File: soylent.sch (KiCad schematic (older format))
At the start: 24 parts, among them J1 DB9_Female, J2 Conn_01x04, J3 Conn_01x04, J4 Conn_02x03_Counter_Clockwise, Q1 BC847BPN, Q2 BC847BPN, U1 ATtiny202-SS, U2 MIC5504-3.3YM5

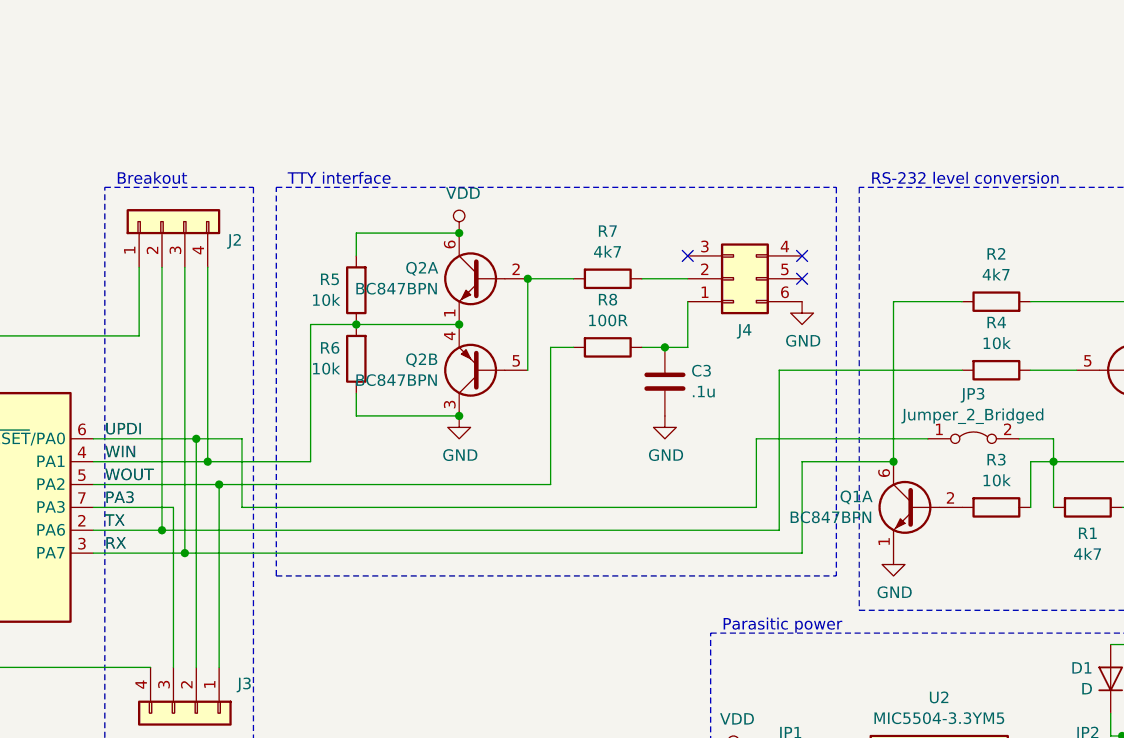
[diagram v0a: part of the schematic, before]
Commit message: Making more room on the schematic
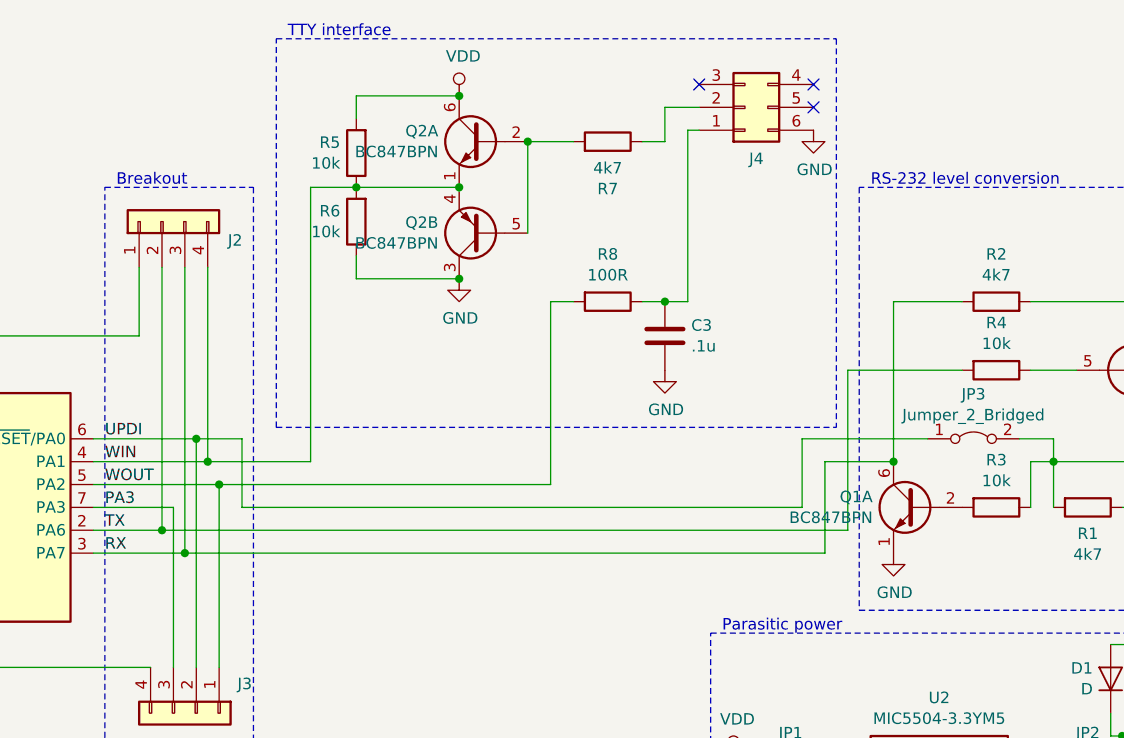
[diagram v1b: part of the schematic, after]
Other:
- moved on the sheet: C3, J4, Q2A, Q2B, R5, R6, R7, R8
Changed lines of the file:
@@
 Connection ~ 3750 3900
 Wire Wire Line
-	6550 4000 6550 3600
-Wire Wire Line
-	6550 3600 6950 3600
+	6650 4000 6650 3600
+Wire Wire Line
+	6650 3600 6950 3600
 Connection ~ 3850 4000
 Wire Wire Line
@@
 Parasitic power
 Wire Notes Line
-	6700 2400 6700 4100
-Wire Notes Line
-	4250 4100 4250 2400
-Wire Wire Line
-	6450 3900 6450 3200
-Wire Wire Line
-	6450 3200 7250 3200
+	6700 1750 6700 3450
+Wire Notes Line
+	4250 3450 4250 1750
+Wire Wire Line
+	6750 3900 6750 3200
+Wire Wire Line
+	6750 3200 7250 3200
 Wire Wire Line
 	7550 3200 7750 3200
-Text Notes 4300 2400 0    50   ~ 0
+Text Notes 4300 1750 0    50   ~ 0
 TTY interface
 $Comp
 L power:GND #PWR0108
 U 1 1 5DEFD9EC
-P 6550 2900
-F 0 "#PWR0108" H 6550 2650 50  0001 C CNN
-F 1 "GND" H 6555 2727 50  0000 C CNN
-F 2 "" H 6550 2900 50  0001 C CNN
-F 3 "" H 6550 2900 50  0001 C CNN
-	1    6550 2900
+P 6600 2150
+F 0 "#PWR0108" H 6600 1900 50  0001 C CNN
+F 1 "GND" H 6605 1977 50  0000 C CNN
+F 2 "" H 6600 2150 50  0001 C CNN
+F 3 "" H 6600 2150 50  0001 C CNN
+	1    6600 2150
 	1    0    0    -1
 $EndComp
@@
 L Device:R R7
 U 1 1 5DEFDFE7
-P 5700 2800
-F 0 "R7" V 5493 2800 50  0000 C CNN
-F 1 "4k7" V 5584 2800 50  0000 C CNN
-F 2 "Resistors_SMD:R_0603_HandSoldering" V 5630 2800 50  0001 C CNN
-F 3 "~" H 5700 2800 50  0001 C CNN
-	1    5700 2800
-	0    1    1    0
+P 5700 2200
+F 0 "R7" V 5493 2200 50  0000 C CNN
+F 1 "4k7" V 5584 2200 50  0000 C CNN
+F 2 "Resistors_SMD:R_0603_HandSoldering" V 5630 2200 50  0001 C CNN
+F 3 "~" H 5700 2200 50  0001 C CNN
+	1    5700 2200
+	0    1    -1   0
 $EndComp
 $Comp
 L Transistor_BJT:BC847BPN Q2
 U 2 1 5DF05573
-P 5150 3200
-F 0 "Q2" H 5341 3154 50  0000 L CNN
-F 1 "BC847BPN" H 5341 3245 50  0000 L CNN
-F 2 "TO_SOT_Packages_SMD:SOT-363_SC-70-6_Handsoldering" H 5350 3300 50  0001 C CNN
-F 3 "https://assets.nexperia.com/documents/data-sheet/BC847BPN.pdf" H 5150 3200 50  0001 C CNN
-	2    5150 3200
+P 5150 2600
+F 0 "Q2" H 5341 2554 50  0000 L CNN
+F 1 "BC847BPN" H 5341 2645 50  0000 L CNN
+F 2 "TO_SOT_Packages_SMD:SOT-363_SC-70-6_Handsoldering" H 5350 2700 50  0001 C CNN
+F 3 "https://assets.nexperia.com/documents/data-sheet/BC847BPN.pdf" H 5150 2600 50  0001 C CNN
+	2    5150 2600
 	-1   0    0    1
 $EndComp
@@
 L Transistor_BJT:BC847BPN Q2
 U 1 1 5DF18897
-P 5150 2800
-F 0 "Q2" H 5341 2846 50  0000 L CNN
-F 1 "BC847BPN" H 5341 2755 50  0000 L CNN
-F 2 "TO_SOT_Packages_SMD:SOT-363_SC-70-6_Handsoldering" H 5350 2900 50  0001 C CNN
-F 3 "https://assets.nexperia.com/documents/data-sheet/BC847BPN.pdf" H 5150 2800 50  0001 C CNN
-	1    5150 2800
+P 5150 2200
+F 0 "Q2" H 5341 2246 50  0000 L CNN
+F 1 "BC847BPN" H 5341 2155 50  0000 L CNN
+F 2 "TO_SOT_Packages_SMD:SOT-363_SC-70-6_Handsoldering" H 5350 2300 50  0001 C CNN
+F 3 "https://assets.nexperia.com/documents/data-sheet/BC847BPN.pdf" H 5150 2200 50  0001 C CNN
+	1    5150 2200
 	-1   0    0    -1
 $EndComp
 Wire Wire Line
-	3750 3900 6450 3900
-Wire Wire Line
-	3850 4000 6550 4000
-Wire Notes Line
-	4250 2400 6700 2400
-Wire Notes Line
-	4250 4100 6700 4100
+	3750 3900 6750 3900
+Wire Wire Line
+	3850 4000 6650 4000
+Wire Notes Line
+	4250 1750 6700 1750
+Wire Notes Line
+	4250 3450 6700 3450
 Wire Wire Line
 	3900 3500 4100 3500
@@
 	4100 3500 4100 3800
 Wire Wire Line
-	4100 3800 6350 3800
-Wire Wire Line
-	6350 3800 6350 3500
-Wire Wire Line
-	6350 3500 7100 3500
+	4100 3800 6550 3800
+Wire Wire Line
+	6550 3800 6550 3500
+Wire Wire Line
+	6550 3500 7100 3500
 Connection ~ 3900 3500
 $Comp
 L power:VDD #PWR0109
 U 1 1 5DF48DE3
-P 5050 2600
-F 0 "#PWR0109" H 5050 2450 50  0001 C CNN
-F 1 "VDD" H 5068 2773 50  0000 C CNN
-F 2 "" H 5050 2600 50  0001 C CNN
-F 3 "" H 5050 2600 50  0001 C CNN
-	1    5050 2600
-	1    0    0    -1
-$EndComp
-$Comp
-L power:GND #PWR0110
-U 1 1 5DF492BB
-P 5050 3400
-F 0 "#PWR0110" H 5050 3150 50  0001 C CNN
-F 1 "GND" H 5055 3227 50  0000 C CNN
-F 2 "" H 5050 3400 50  0001 C CNN
-F 3 "" H 5050 3400 50  0001 C CNN
-	1    5050 3400
-	1    0    0    -1
-$EndComp
-Wire Wire Line
-	5050 3000 4600 3000
-Connection ~ 5050 3000
-Wire Wire Line
-	5350 3200 5350 2800
-Wire Wire Line
-	5350 2800 5550 2800
-Connection ~ 5350 2800
-Wire Wire Line
-	5850 2800 6050 2800
+P 5050 2000
+F 0 "#PWR0109" H 5050 1850 50  0001 C CNN
+F 1 "VDD" H 5068 2173 50  0000 C CNN
+F 2 "" H 5050 2000 50  0001 C CNN
+F 3 "" H 5050 2000 50  0001 C CNN
+	1    5050 2000
+	1    0    0    -1
+$EndComp
+Wire Wire Line
+	5050 2400 4600 2400
+Connection ~ 5050 2400
+Wire Wire Line
+	5350 2600 5350 2200
+Wire Wire Line
+	5350 2200 5550 2200
+Connection ~ 5350 2200
 $Comp
 L Device:R R5
 U 1 1 5DF5183F
-P 4600 2850
-F 0 "R5" H 4670 2804 50  0000 L CNN
-F 1 "10k" H 4670 2895 50  0000 L CNN
-F 2 "Resistors_SMD:R_0603_HandSoldering" V 4530 2850 50  0001 C CNN
-F 3 "~" H 4600 2850 50  0001 C CNN
-	1    4600 2850
+P 4600 2250
+F 0 "R5" H 4670 2204 50  0000 L CNN
+F 1 "10k" H 4670 2295 50  0000 L CNN
+F 2 "Resistors_SMD:R_0603_HandSoldering" V 4530 2250 50  0001 C CNN
+F 3 "~" H 4600 2250 50  0001 C CNN
+	1    4600 2250
 	-1   0    0    1
 $EndComp
@@
 L Device:R R6
 U 1 1 5DF52A36
-P 4600 3150
-F 0 "R6" H 4670 3104 50  0000 L CNN
-F 1 "10k" H 4670 3195 50  0000 L CNN
-F 2 "Resistors_SMD:R_0603_HandSoldering" V 4530 3150 50  0001 C CNN
-F 3 "~" H 4600 3150 50  0001 C CNN
-	1    4600 3150
+P 4600 2550
+F 0 "R6" H 4670 2504 50  0000 L CNN
+F 1 "10k" H 4670 2595 50  0000 L CNN
+F 2 "Resistors_SMD:R_0603_HandSoldering" V 4530 2550 50  0001 C CNN
+F 3 "~" H 4600 2550 50  0001 C CNN
+	1    4600 2550
 	-1   0    0    1
 $EndComp
-Connection ~ 4600 3000
-Wire Wire Line
-	5050 2600 4600 2600
-Wire Wire Line
-	4600 2600 4600 2700
-Connection ~ 5050 2600
-Wire Wire Line
-	5050 3400 4600 3400
-Wire Wire Line
-	4600 3400 4600 3300
-Connection ~ 5050 3400
+Connection ~ 4600 2400
+Wire Wire Line
+	5050 2000 4600 2000
+Wire Wire Line
+	4600 2000 4600 2100
+Connection ~ 5050 2000
+Wire Wire Line
+	5050 2800 4600 2800
+Wire Wire Line
+	4600 2800 4600 2700
 Wire Wire Line
 	8350 3700 8350 4400
@@
 	8250 4250 8250 2400
 Wire Wire Line
-	4400 3000 4600 3000
-NoConn ~ 6050 2700
-NoConn ~ 6550 2700
-NoConn ~ 6550 2800
+	4400 2400 4600 2400
+NoConn ~ 6100 1950
+NoConn ~ 6600 1950
+NoConn ~ 6600 2050
 $Comp
 L Connector_Generic:Conn_02x03_Counter_Clockwise J4
 U 1 1 5DDE85A2
-P 6250 2800
-F 0 "J4" H 6300 3025 50  0000 C CNN
-F 1 "Conn_02x03_Counter_Clockwise" V 6345 2980 50  0001 L CNN
-F 2 "Pin_Headers:Pin_Header_Straight_2x03_Pitch2.54mm" H 6250 2800 50  0001 C CNN
-F 3 "~" H 6250 2800 50  0001 C CNN
-	1    6250 2800
+P 6300 2050
+F 0 "J4" H 6350 2275 50  0000 C CNN
+F 1 "Conn_02x03_Counter_Clockwise" V 6395 2230 50  0001 L CNN
+F 2 "Pin_Headers:Pin_Header_Straight_2x03_Pitch2.54mm" H 6300 2050 50  0001 C CNN
+F 3 "~" H 6300 2050 50  0001 C CNN
+	1    6300 2050
 	1    0    0    1
 $EndComp
@@
 	3950 3600 4400 3600
 Connection ~ 3950 3600
-Wire Wire Line
-	4400 3600 4400 3000
 Connection ~ 4000 3700
 $Comp
 L Device:R R8
 U 1 1 5DFD8224
-P 5700 3100
-F 0 "R8" V 5493 3100 50  0000 C CNN
-F 1 "100R" V 5584 3100 50  0000 C CNN
-F 2 "Resistors_SMD:R_0603_HandSoldering" V 5630 3100 50  0001 C CNN
-F 3 "~" H 5700 3100 50  0001 C CNN
-	1    5700 3100
+P 5700 2900
+F 0 "R8" V 5493 2900 50  0000 C CNN
+F 1 "100R" V 5584 2900 50  0000 C CNN
+F 2 "Resistors_SMD:R_0603_HandSoldering" V 5630 2900 50  0001 C CNN
+F 3 "~" H 5700 2900 50  0001 C CNN
+	1    5700 2900
 	0    1    1    0
 $EndComp
-Wire Wire Line
-	5450 3700 5450 3100
-Wire Wire Line
-	5450 3100 5550 3100
-Wire Wire Line
-	4000 3700 5450 3700
 $Comp
 L Device:C C3
 U 1 1 5DFEE336
-P 5950 3250
-F 0 "C3" H 6065 3296 50  0000 L CNN
-F 1 ".1u" H 6065 3205 50  0000 L CNN
-F 2 "Capacitor_SMD:C_0603_1608Metric_Pad1.05x0.95mm_HandSolder" H 5988 3100 50  0001 C CNN
-F 3 "~" H 5950 3250 50  0001 C CNN
-	1    5950 3250
+P 5950 3050
+F 0 "C3" H 6065 3096 50  0000 L CNN
+F 1 ".1u" H 6065 3005 50  0000 L CNN
+F 2 "Capacitor_SMD:C_0603_1608Metric_Pad1.05x0.95mm_HandSolder" H 5988 2900 50  0001 C CNN
+F 3 "~" H 5950 3050 50  0001 C CNN
+	1    5950 3050
 	1    0    0    -1
 $EndComp
@@
 L power:GND #PWR0111
 U 1 1 5DFEEE43
-P 5950 3400
-F 0 "#PWR0111" H 5950 3150 50  0001 C CNN
-F 1 "GND" H 5955 3227 50  0000 C CNN
-F 2 "" H 5950 3400 50  0001 C CNN
-F 3 "" H 5950 3400 50  0001 C CNN
-	1    5950 3400
-	1    0    0    -1
-$EndComp
-Wire Wire Line
-	5850 3100 5950 3100
-Wire Wire Line
-	5950 3100 6050 3100
-Wire Wire Line
-	6050 3100 6050 2900
-Connection ~ 5950 3100
+P 5950 3200
+F 0 "#PWR0111" H 5950 2950 50  0001 C CNN
+F 1 "GND" H 5955 3027 50  0000 C CNN
+F 2 "" H 5950 3200 50  0001 C CNN
+F 3 "" H 5950 3200 50  0001 C CNN
+	1    5950 3200
+	1    0    0    -1
+$EndComp
+Wire Wire Line
+	5850 2900 5950 2900
 Wire Wire Line
 	7500 3500 7650 3500
@@
 Wire Wire Line
 	7650 3600 7650 3800
+Wire Wire Line
+	5850 2200 5950 2200
+Wire Wire Line
+	5950 2200 5950 2050
+Wire Wire Line
+	5950 2050 6100 2050
+Wire Wire Line
+	4400 2400 4400 3600
+Wire Wire Line
+	5950 2900 6050 2900
+Wire Wire Line
+	6050 2900 6050 2150
+Wire Wire Line
+	6050 2150 6100 2150
+Connection ~ 5950 2900
+Connection ~ 5050 2800
+$Comp
+L power:GND #PWR0110
+U 1 1 5DF492BB
+P 5050 2800
+F 0 "#PWR0110" H 5050 2550 50  0001 C CNN
+F 1 "GND" H 5055 2627 50  0000 C CNN
+F 2 "" H 5050 2800 50  0001 C CNN
+F 3 "" H 5050 2800 50  0001 C CNN
+	1    5050 2800
+	1    0    0    -1
+$EndComp
+Wire Wire Line
+	5450 2900 5550 2900
+Wire Wire Line
+	4000 3700 5450 3700
+Wire Wire Line
+	5450 3700 5450 2900
 $EndSCHEMATC
